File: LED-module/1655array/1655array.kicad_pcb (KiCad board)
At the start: 2 copper layers, 22 x 94 mm, 35 parts, among them J1 Conn_01x04, J2 Conn_02x02_Counter_Clockwise, J3 Conn_02x02_Counter_Clockwise, J4 Conn_02x02_Counter_Clockwise, J5 Conn_02x02_Counter_Clockwise

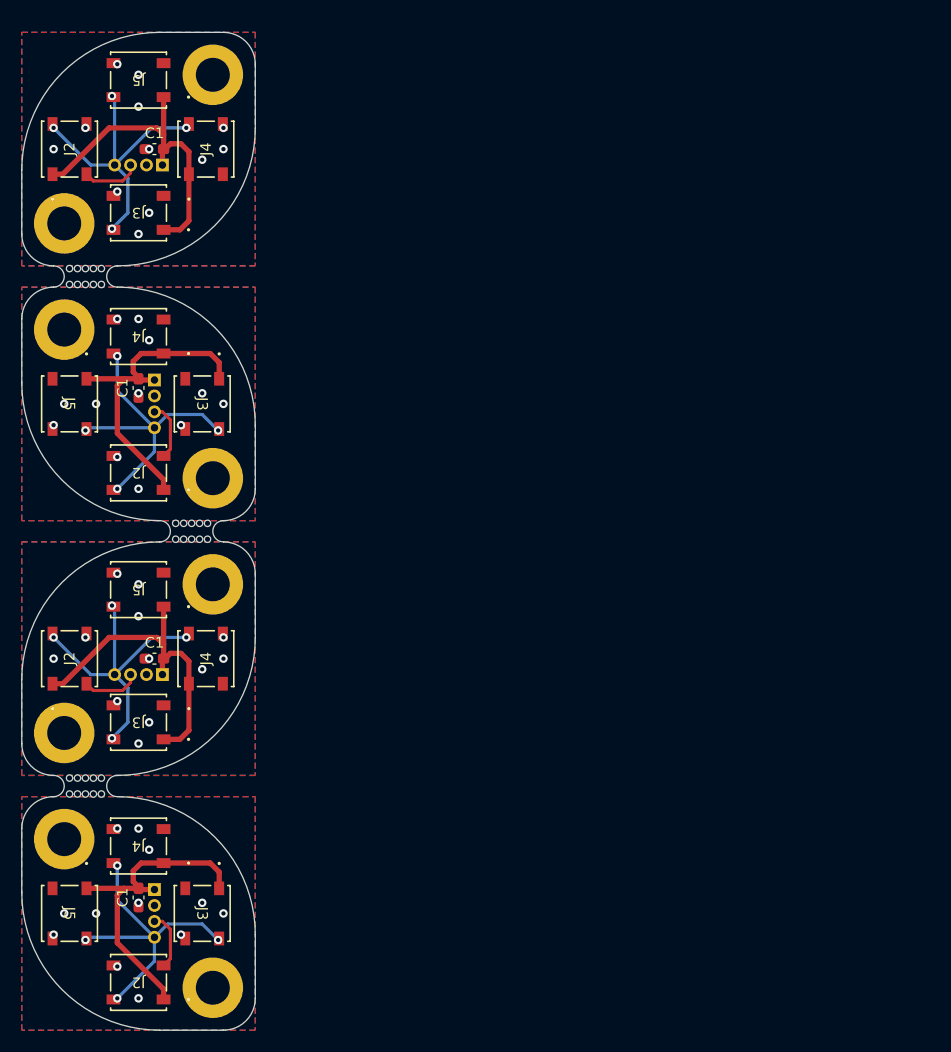
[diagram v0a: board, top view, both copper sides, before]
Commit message: expand
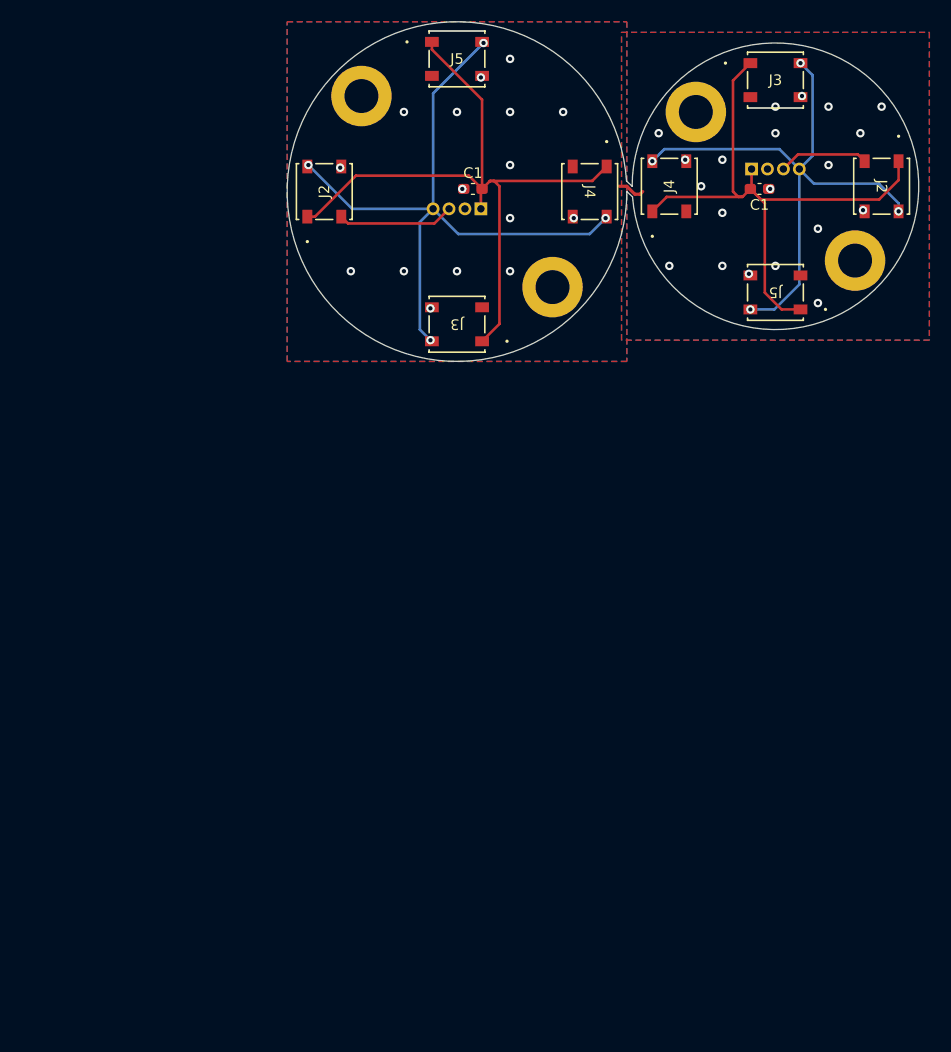
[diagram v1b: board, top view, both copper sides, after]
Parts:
- removed the C1 at (150.0, 136.5)
- removed the C1 at (150.0, 88.5)
- removed the C1 at (151.5, 114.0)
- removed the H1 at (157.0, 145.0)
- removed the H1 at (143.0, 121.0)
- removed the H1 at (157.0, 97.0)
- removed the H2 at (143.0, 131.0)
- removed the H2 at (157.0, 107.0)
- removed the H2 at (143.0, 83.0)
- removed the J1 at (151.5, 90.0)
- removed the J1 at (151.5, 138.0)
- removed the J1 at (150.0, 115.5)
- removed the J2 at (143.5, 114.0)
- removed the J2 at (150.0, 144.5)
- removed the J2 at (150.0, 96.5)
- removed the J3 at (156.0, 138.0)
- removed the J3 at (156.0, 90.0)
- removed the J3 at (150.0, 120.0)
- removed the J4 at (156.3, 114.0)
- removed the J4 at (150.0, 131.7)
- removed the J4 at (150.0, 83.7)
- removed the J5 at (143.5, 138.0)
- removed the J5 at (143.5, 90.0)
- removed the J5 at (150.0, 107.5)
- removed REF** (x3): stamphole_2x5, LED-module:stamphole_2x5
- added C1: C, Capacitor_SMD:C_0603_1608Metric_Pad1.08x0.95mm_HandSolder, F.Cu at (208.5, 69.8)
- added H1: MountingHole, MountingHole:MountingHole_3.2mm_M3_ISO7380_Pad, F.Cu at (202.5, 62.5)
- added H2: MountingHole, MountingHole:MountingHole_3.2mm_M3_ISO7380_Pad, F.Cu at (217.5, 76.5)
- added J1: Conn_01x04, LED-module:JST_S4B-ZR_LF__SN_, B.Cu at (210.0, 67.9)
- added J2: Conn_02x02_Counter_Clockwise, LED-module:LED_2758_ADA, F.Cu at (220.0, 69.5)
- added J3: Conn_02x02_Counter_Clockwise, LED-module:LED_2758_ADA, F.Cu at (210.0, 59.5)
- added J4: Conn_02x02_Counter_Clockwise, LED-module:LED_2758_ADA, F.Cu at (200.0, 69.5)
- added J5: Conn_02x02_Counter_Clockwise, LED-module:LED_2758_ADA, F.Cu at (210.0, 79.5)
- moved H1 46.4 mm to (189.0, 79.0)
- moved J4 36.4 mm to (192.5, 70.0), turned to -90 degrees
- moved J3 31.8 mm to (180.0, 82.5)
- moved J1 30.3 mm to (180.0, 71.6)
- moved C1 30.2 mm to (181.5, 69.8)
- moved J5 30.1 mm to (180.0, 57.5), turned to 0 degrees
- moved J2 24.3 mm to (167.5, 70.0)
- moved H2 14.1 mm to (171.0, 61.0)
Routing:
- net (no net): track 0.00 -> 2.66 mm
- net /DOUT: track 21.9 -> 19.5 mm
- net +5V: track 124.5 -> 122.5 mm
- net /DIN: track 116.6 -> 116.2 mm, vias 16 -> 8
- net GND: vias 48 -> 36
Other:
- board size 22 x 94 mm -> 59.5 x 32 mm
- board text removed: "MountingHole"
